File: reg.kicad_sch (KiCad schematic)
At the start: 20 parts, among them Q2 NJVMJD45H11T4G, Q3 PNP, U1 AD817

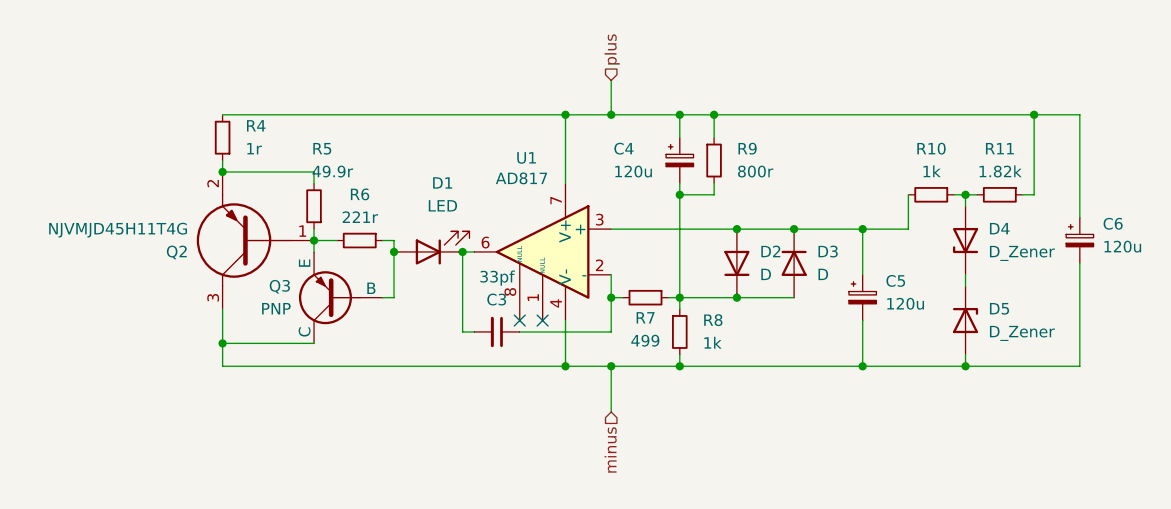
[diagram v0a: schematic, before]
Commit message: pretty neat neg needs testing
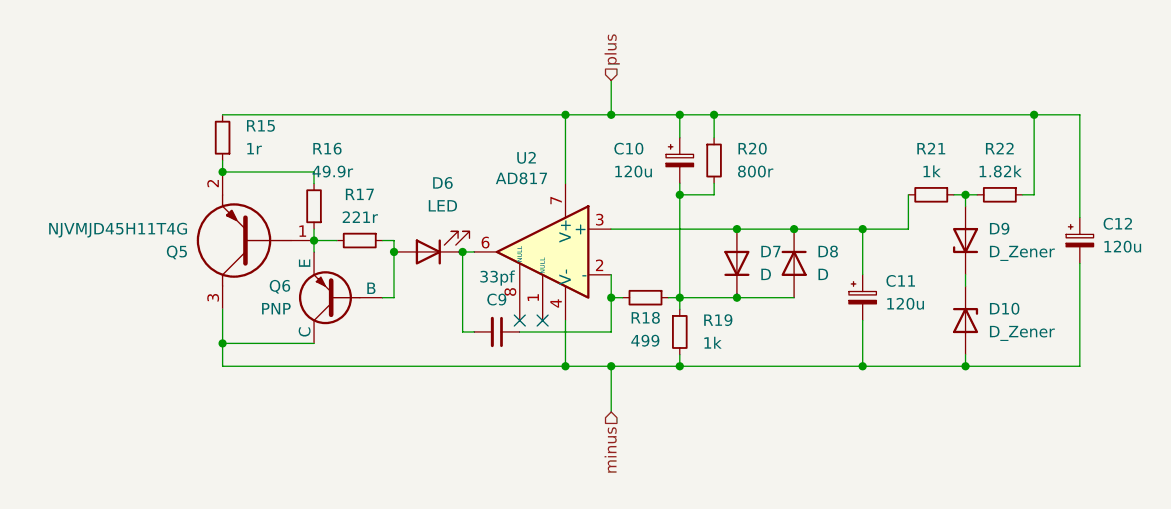
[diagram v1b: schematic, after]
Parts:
- renumbered C4 to C10, C5 to C11, C6 to C12, C3 to C9, D5 to D10, D1 to D6, D2 to D7, D3 to D8, D4 to D9, Q2 to Q5, Q3 to Q6, R4 to R15, R5 to R16, R6 to R17, R7 to R18, R8 to R19, R9 to R20, R10 to R21, R11 to R22, U1 to U2
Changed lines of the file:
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@@
 		(dnp no)
 		(fields_autoplaced yes)
-		(property "Reference" "R8"
+		(property "Reference" "R19"
 			(at 189.23 118.1099 0)
 			(effects
@@
 		(dnp no)
 		(fields_autoplaced yes)
-		(property "Reference" "R4"
+		(property "Reference" "R15"
 			(at 138.43 96.5199 0)
 			(effects
@@
 		(dnp no)
 		(fields_autoplaced yes)
-		(property "Reference" "D4"
+		(property "Reference" "D9"
 			(at 220.98 107.9499 90)
 			(effects
@@
 		(on_board yes)
 		(dnp no)
-		(property "Reference" "C3"
+		(property "Reference" "C9"
 			(at 166.37 115.824 90)
 			(effects
@@
 		(on_board yes)
 		(dnp no)
-		(property "Reference" "Q2"
+		(property "Reference" "Q5"
 			(at 132.08 110.4901 0)
 			(effects
@@
 		(dnp no)
 		(fields_autoplaced yes)
-		(property "Reference" "R11"
+		(property "Reference" "R22"
 			(at 222.25 99.06 90)
 			(effects
@@
 		(on_board yes)
 		(dnp no)
-		(property "Reference" "C6"
+		(property "Reference" "C12"
 			(at 233.68 107.4038 0)
 			(effects
@@
 		(dnp no)
 		(fields_autoplaced yes)
-		(property "Reference" "C5"
+		(property "Reference" "C11"
 			(at 209.55 113.7538 0)
 			(effects
@@
 		(dnp no)
 		(fields_autoplaced yes)
-		(property "Reference" "Q3"
+		(property "Reference" "Q6"
 			(at 143.51 114.2999 0)
 			(effects
@@
 		(dnp no)
 		(fields_autoplaced yes)
-		(property "Reference" "R6"
+		(property "Reference" "R17"
 			(at 151.13 104.14 90)
 			(effects
@@
 		(dnp no)
 		(fields_autoplaced yes)
-		(property "Reference" "D1"
+		(property "Reference" "D6"
 			(at 160.3375 102.87 0)
 			(effects
@@
 		(dnp no)
 		(fields_autoplaced yes)
-		(property "Reference" "D3"
+		(property "Reference" "D8"
 			(at 201.93 110.4899 90)
 			(effects
@@
 		(dnp no)
 		(fields_autoplaced yes)
-		(property "Reference" "R10"
+		(property "Reference" "R21"
 			(at 214.63 99.06 90)
 			(effects
@@
 		(on_board yes)
 		(dnp no)
-		(property "Reference" "C4"
+		(property "Reference" "C10"
 			(at 179.324 99.06 0)
 			(effects
@@
 		(dnp no)
 		(fields_autoplaced yes)
-		(property "Reference" "R9"
+		(property "Reference" "R20"
 			(at 193.04 99.0599 0)
 			(effects
@@
 		(on_board yes)
 		(dnp no)
-		(property "Reference" "R5"
+		(property "Reference" "R16"
 			(at 145.796 99.06 0)
 			(effects
@@
 		(on_board yes)
 		(dnp no)
-		(property "Reference" "R7"
+		(property "Reference" "R18"
 			(at 182.88 117.856 90)
 			(effects
@@
 		(dnp no)
 		(fields_autoplaced yes)
-		(property "Reference" "D5"
+		(property "Reference" "D10"
 			(at 220.98 116.8399 90)
 			(effects
@@
 		(on_board yes)
 		(dnp no)
-		(property "Reference" "U1"
+		(property "Reference" "U2"
 			(at 169.672 100.076 0)
 			(effects
@@
 		(dnp no)
 		(fields_autoplaced yes)
-		(property "Reference" "D2"
+		(property "Reference" "D7"
 			(at 195.58 110.4899 90)
 			(effects
